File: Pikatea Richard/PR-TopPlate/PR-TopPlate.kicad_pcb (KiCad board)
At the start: 2 copper layers, 62 x 136.7 mm, 7 parts, among them SW1 Rotary_Encoder_Switch, SW2 Rotary_Encoder_Switch

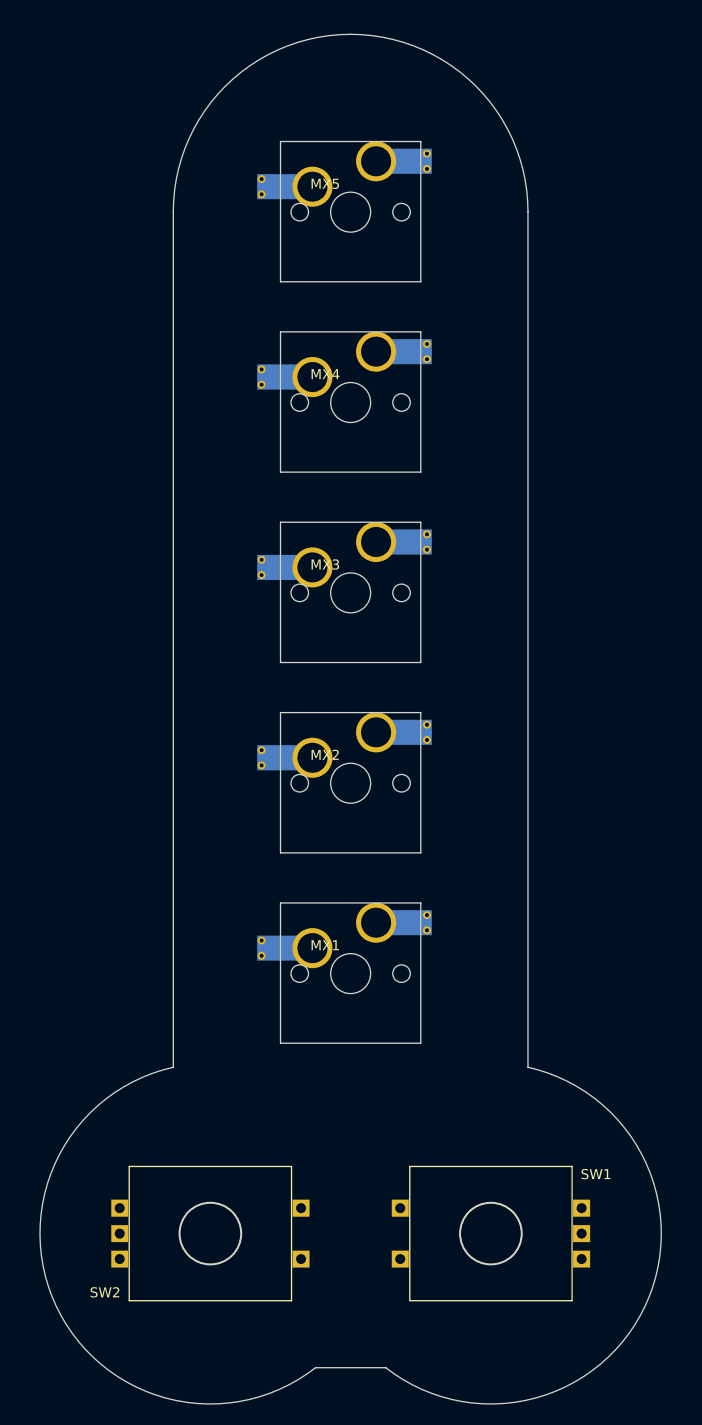
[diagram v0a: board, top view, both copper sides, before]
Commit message: updated footprints added gerbers
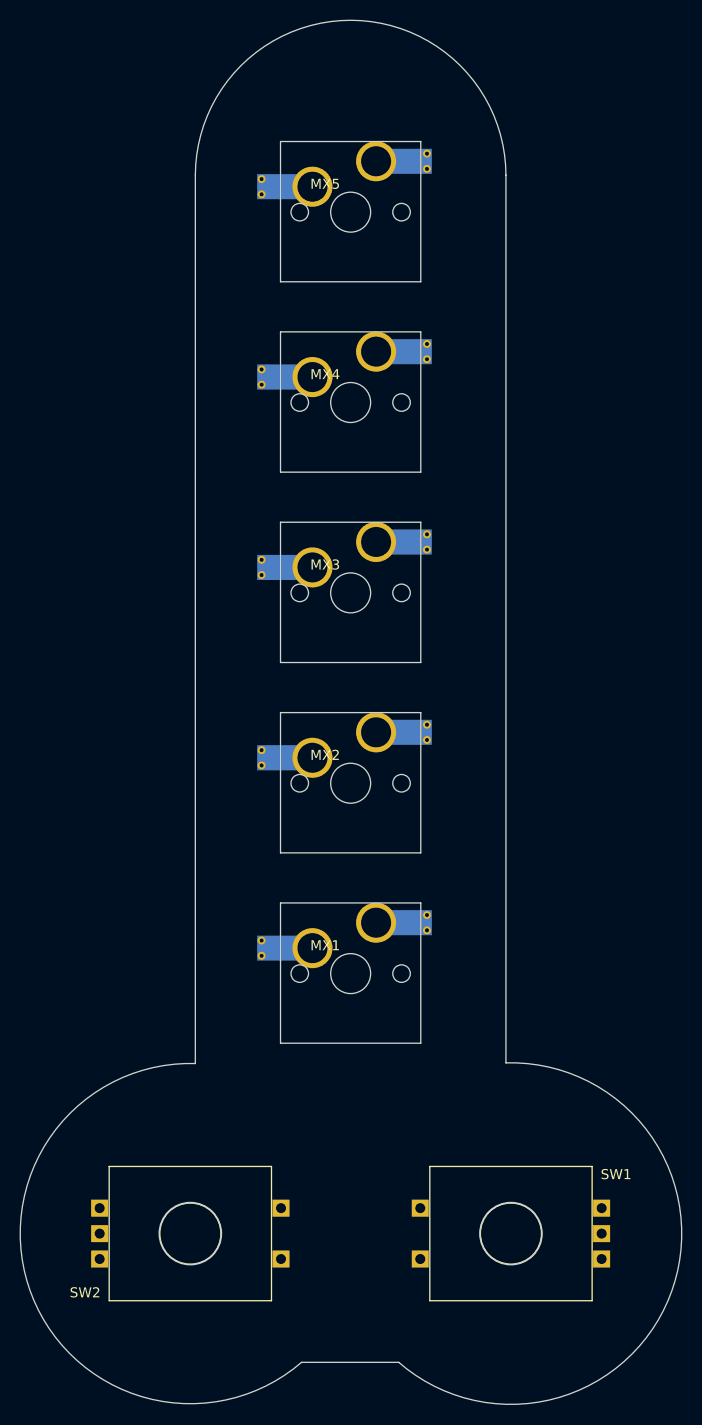
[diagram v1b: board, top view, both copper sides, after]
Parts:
- moved SW1 2.00 mm to (155.0, 100.0)
- moved SW2 2.00 mm to (123.0, 100.0)
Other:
- board size 62 x 136.7 mm -> 66 x 138.1 mm
